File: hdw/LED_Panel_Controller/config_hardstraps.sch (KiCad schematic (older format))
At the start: 19 parts, among them J1201 PIC_UART, J1202 WIFI_UART, J1203 I2C, J1204 WIFI_SPI, J1205 SD_SPI, J1206 FLASH_SPI, U1201 MCP9804

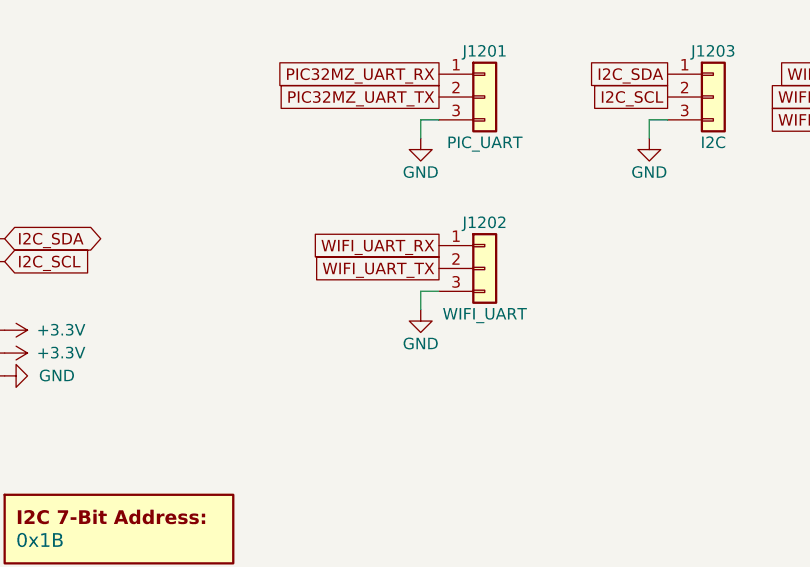
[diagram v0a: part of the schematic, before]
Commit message: having a mid-project crisis
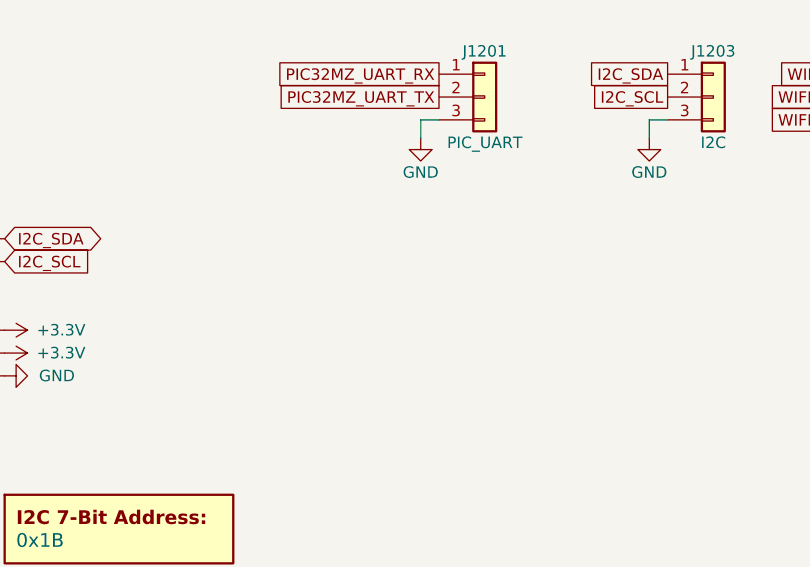
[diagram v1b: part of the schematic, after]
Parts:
- removed J1202: WIFI_UART, Connector_PinHeader_2.54mm:PinHeader_1x03_P2.54mm_Vertical, symbol Connector_Generic:Conn_01x03
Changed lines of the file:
@@
 	0    1    -1   0
 $EndComp
-Wire Wire Line
-	4740 5870 4820 5870
-Wire Wire Line
-	4740 5950 4740 5870
-$Comp
-L power:GND #PWR01215
-U 1 1 6022B183
-P 4740 5950
-F 0 "#PWR01215" H 4740 5700 50  0001 C CNN
-F 1 "GND" H 4740 5800 50  0000 C CNN
-F 2 "" H 4740 5950 50  0001 C CNN
-F 3 "" H 4740 5950 50  0001 C CNN
-	1    4740 5950
-	1    0    0    -1
-$EndComp
-$Comp
-L Connector_Generic:Conn_01x03 J1202
-U 1 1 6022AEF7
-P 5020 5770
-F 0 "J1202" H 5020 5970 50  0000 C CNN
-F 1 "WIFI_UART" H 5020 5570 50  0000 C CNN
-F 2 "Connector_PinHeader_2.54mm:PinHeader_1x03_P2.54mm_Vertical" H 5020 5770 50  0001 C CNN
-F 3 "~" H 5020 5770 50  0001 C CNN
-F 4 "DNP" H 5020 5770 50  0001 C CNN "Configuration"
-	1    5020 5770
-	1    0    0    -1
-$EndComp
-Text GLabel 4820 5770 0    50   UnSpc ~ 0
-WIFI_UART_TX
-Text GLabel 4820 5670 0    50   UnSpc ~ 0
-WIFI_UART_RX
 Text GLabel 4820 5020 0    50   UnSpc ~ 0
 PIC32MZ_UART_TX
